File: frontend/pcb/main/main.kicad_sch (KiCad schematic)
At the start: 33 parts, among them J1 Ext, J2 Conn_01x02, J3 Conn_01x09, J4 Debug, J5 RS485, J6 Conn_01x04, J7 Conn_01x02, Q1 MMBT3904, Q2 MMBT3904, U1 ESP32-WROOM-32, U2 AP1117-33, U3 MAX485E

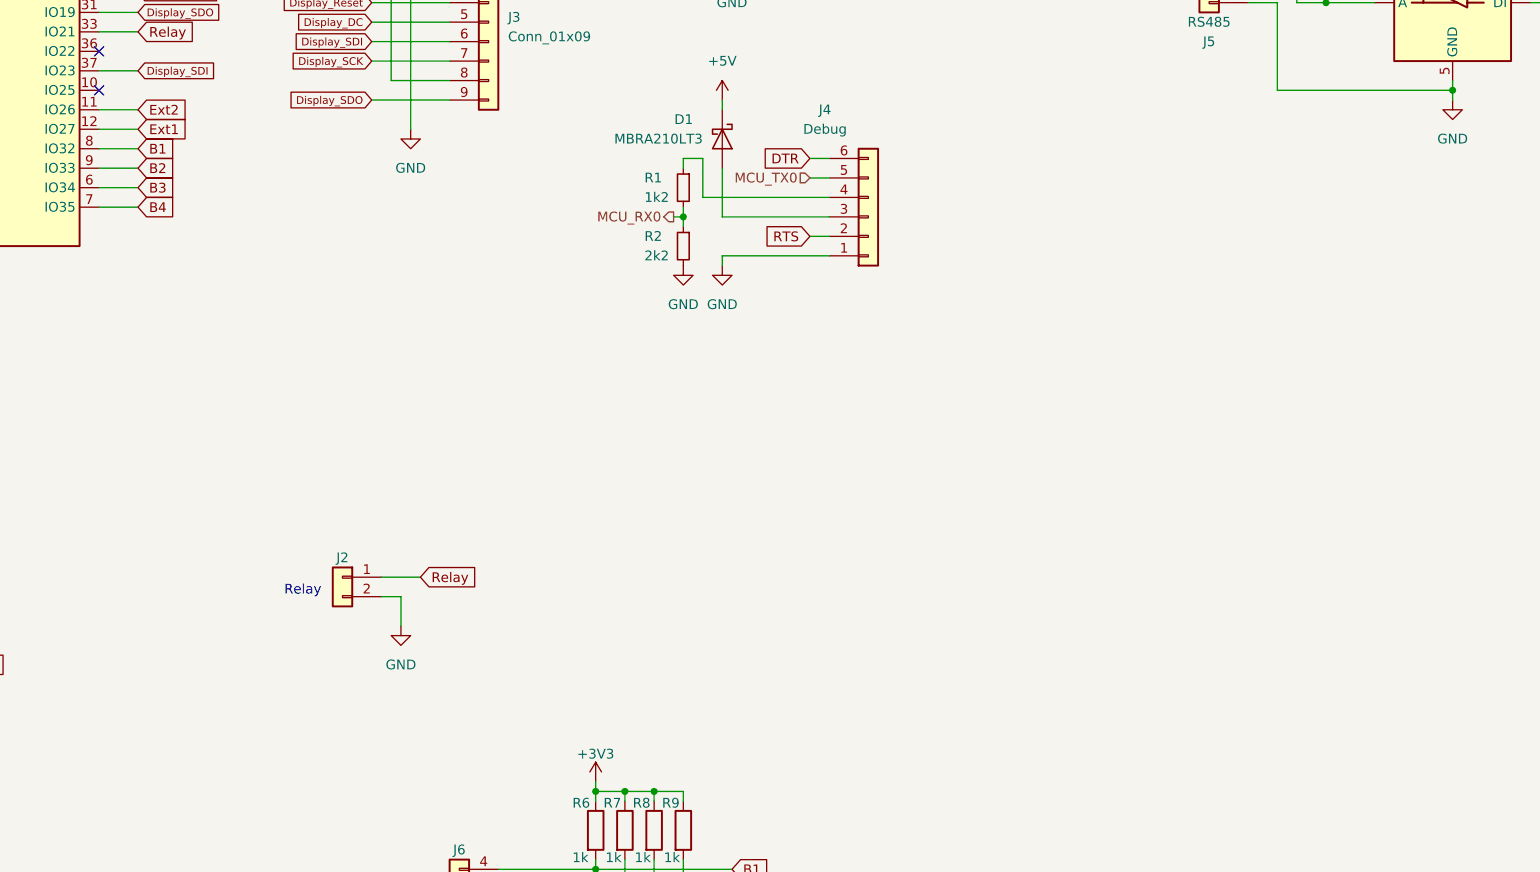
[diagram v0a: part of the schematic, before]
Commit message: Finish relay board.
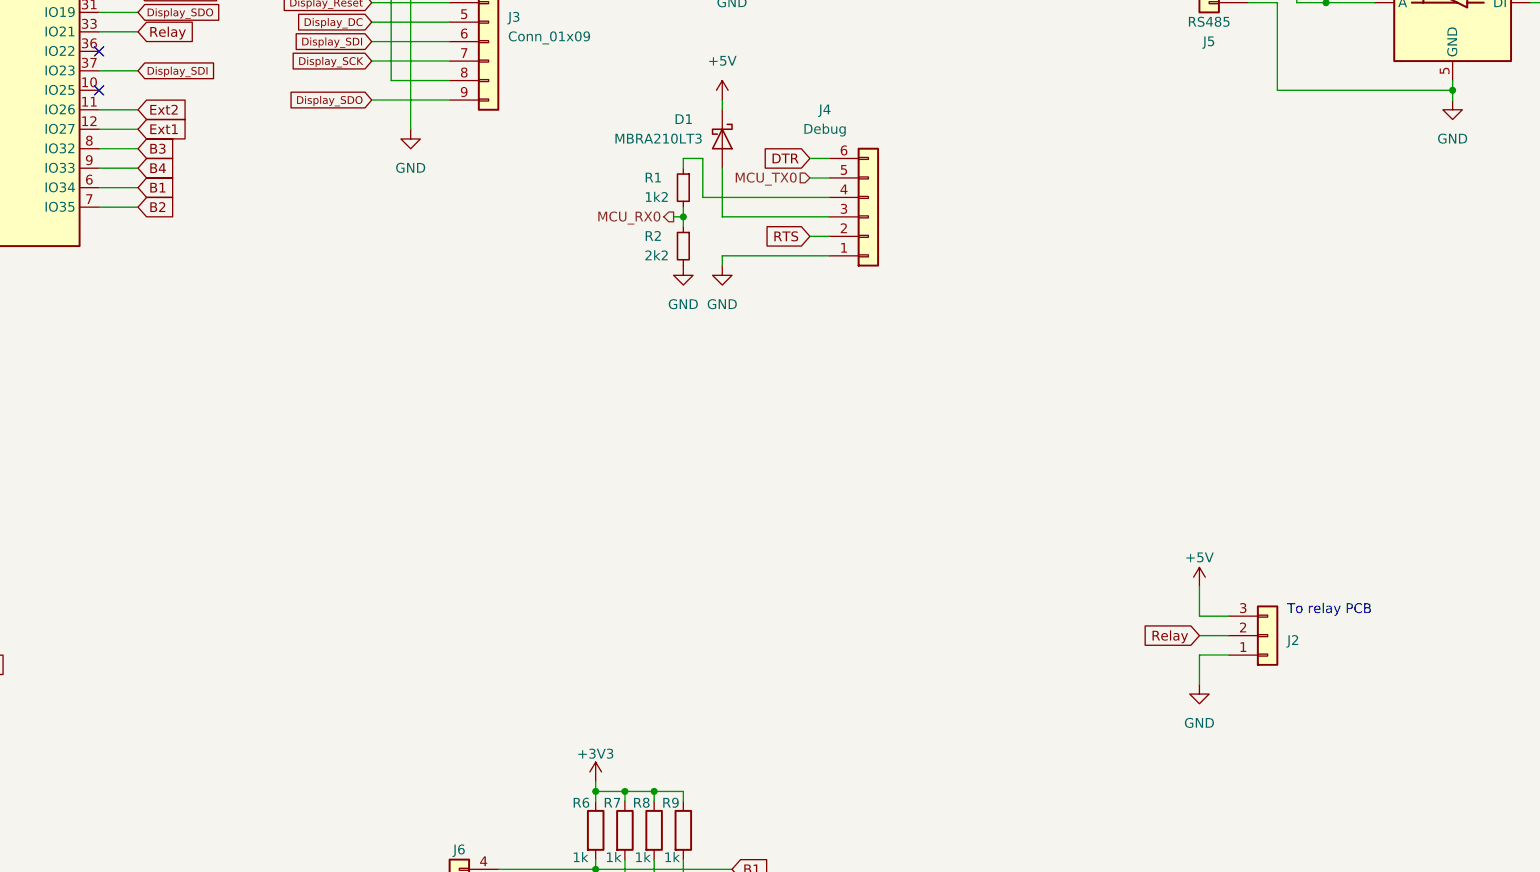
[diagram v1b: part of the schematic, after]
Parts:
- removed J2: Conn_01x02, Connector_JST:JST_XH_B2B-XH-A_1x02_P2.50mm_Vertical, symbol Connector_Generic:Conn_01x02
- added J2: Conn_01x03, Connector_PinHeader_2.54mm:PinHeader_1x03_P2.54mm_Vertical, symbol Connector_Generic:Conn_01x03
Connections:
- net +5V: now also J2.3 (Pin_3)
- net B1: now also U1.6 (IO34); no longer U1.8 (IO32)
- net B2: now also U1.7 (IO35); no longer U1.9 (IO33)
- net B3: now also U1.8 (IO32); no longer U1.6 (IO34)
- net B4: now also U1.9 (IO33); no longer U1.7 (IO35)
- net GND: now also J2.1 (Pin_1)
- net Relay: now also J2.2 (Pin_2)
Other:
- note added: "To relay PCB"
- note removed: "Relay"
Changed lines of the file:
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@@
+    (stroke (width 0) (type default))
+  )
+  (wire (pts (xy 232.41 146.05) (xy 232.41 149.86))
     (stroke (width 0) (type default))
   )
@@
     (stroke (width 0) (type default))
   )
+  (wire (pts (xy 232.41 137.16) (xy 232.41 140.97))
+    (stroke (width 0) (type default))
+  )
   (wire (pts (xy 153.67 173.99) (xy 171.45 173.99))
     (stroke (width 0) (type default))
@@
     (stroke (width 0) (type default))
   )
-  (wire (pts (xy 125.73 138.43) (xy 128.27 138.43))
-    (stroke (width 0) (type default))
-  )
   (wire (pts (xy 25.4 173.99) (xy 25.4 177.8))
     (stroke (width 0) (type default))
@@
     (stroke (width 0) (type default))
   )
-  (wire (pts (xy 128.27 138.43) (xy 128.27 142.24))
-    (stroke (width 0) (type default))
-  )
   (wire (pts (xy 88.9 46.99) (xy 93.98 46.99))
     (stroke (width 0) (type default))
   )
-  (wire (pts (xy 125.73 135.89) (xy 130.81 135.89))
-    (stroke (width 0) (type default))
-  )
   (wire (pts (xy 181.61 44.45) (xy 181.61 45.72))
     (stroke (width 0) (type default))
@@
     (stroke (width 0) (type default))
   )
+  (wire (pts (xy 232.41 143.51) (xy 236.22 143.51))
+    (stroke (width 0) (type default))
+  )
   (wire (pts (xy 58.42 147.32) (xy 68.58 147.32))
     (stroke (width 0) (type default))
@@
     (stroke (width 0) (type default))
   )
+  (wire (pts (xy 232.41 140.97) (xy 236.22 140.97))
+    (stroke (width 0) (type default))
+  )
   (wire (pts (xy 171.45 181.61) (xy 165.1 181.61))
     (stroke (width 0) (type default))
@@
     (stroke (width 0) (type default))
   )
+  (wire (pts (xy 236.22 146.05) (xy 232.41 146.05))
+    (stroke (width 0) (type default))
+  )
   (wire (pts (xy 281.94 69.85) (xy 281.94 71.12))
     (stroke (width 0) (type default))
@@
   (wire (pts (xy 88.9 31.75) (xy 91.44 31.75))
     (stroke (width 0) (type default))
-  )
-  (text "Relay" (exclude_from_sim no)
- (at 113.03 138.43 0)
-    (effects (font (size 1.27 1.27)) (justify left bottom))
   )
   (text "MSP4020" (exclude_from_sim no)
@@
     (effects (font (size 1.27 1.27)) (justify left bottom))
   )
-  (global_label "B2" (shape input) (at 93.98 82.55 0) (fields_autoplaced)
-    (effects (font (size 1.27 1.27)) (justify left))
-    (property "Intersheetrefs" "${INTERSHEET_REFS}" (at 99.3653 82.55 0)
+  (text "To relay PCB" (exclude_from_sim no)
+ (at 243.84 140.97 0)
+    (effects (font (size 1.27 1.27)) (justify left bottom))
+  )
+  (global_label "B2" (shape input) (at 93.98 87.63 0) (fields_autoplaced)
+    (effects (font (size 1.27 1.27)) (justify left))
+    (property "Intersheetrefs" "${INTERSHEET_REFS}" (at 99.3653 87.63 0)
       (effects (font (size 1.27 1.27)) (justify left) hide)
     )
@@
     )
   )
-  (global_label "B4" (shape input) (at 93.98 87.63 0) (fields_autoplaced)
-    (effects (font (size 1.27 1.27)) (justify left))
-    (property "Intersheetrefs" "${INTERSHEET_REFS}" (at 99.3653 87.63 0)
+  (global_label "B4" (shape input) (at 93.98 82.55 0) (fields_autoplaced)
+    (effects (font (size 1.27 1.27)) (justify left))
+    (property "Intersheetrefs" "${INTERSHEET_REFS}" (at 99.3653 82.55 0)
       (effects (font (size 1.27 1.27)) (justify left) hide)
     )
@@
     )
   )
-  (global_label "B3" (shape input) (at 93.98 85.09 0) (fields_autoplaced)
+  (global_label "B3" (shape input) (at 93.98 80.01 0) (fields_autoplaced)
+    (effects (font (size 1.27 1.27)) (justify left))
+    (property "Intersheetrefs" "${INTERSHEET_REFS}" (at 99.3653 80.01 0)
+      (effects (font (size 1.27 1.27)) (justify left) hide)
+    )
+  )
+  (global_label "B1" (shape input) (at 93.98 85.09 0) (fields_autoplaced)
     (effects (font (size 1.27 1.27)) (justify left))
     (property "Intersheetrefs" "${INTERSHEET_REFS}" (at 99.3653 85.09 0)
-      (effects (font (size 1.27 1.27)) (justify left) hide)
-    )
-  )
-  (global_label "B1" (shape input) (at 93.98 80.01 0) (fields_autoplaced)
-    (effects (font (size 1.27 1.27)) (justify left))
-    (property "Intersheetrefs" "${INTERSHEET_REFS}" (at 99.3653 80.01 0)
       (effects (font (size 1.27 1.27)) (justify left) hide)
     )
@@
     )
   )
-  (global_label "Relay" (shape input) (at 130.81 135.89 0) (fields_autoplaced)
-    (effects (font (size 1.27 1.27)) (justify left))
-    (property "Intersheetrefs" "${INTERSHEET_REFS}" (at 138.8562 135.89 0)
-      (effects (font (size 1.27 1.27)) (justify left) hide)
-    )
-  )
   (global_label "BOOT" (shape input) (at 91.44 29.21 0) (fields_autoplaced)
     (effects (font (size 1.27 1.27)) (justify left))
@@
     (property "Intersheetrefs" "${INTERSHEET_REFS}" (at 176.5331 178.9906 0)
       (effects (font (size 1.27 1.27)) (justify left) hide)
+    )
+  )
+  (global_label "Relay" (shape input) (at 232.41 143.51 180) (fields_autoplaced)
+    (effects (font (size 1.27 1.27)) (justify right))
+    (property "Intersheetrefs" "${INTERSHEET_REFS}" (at 224.3638 143.51 0)
+      (effects (font (size 1.27 1.27)) (justify right) hide)
     )
   )
@@
     )
   )
-  (symbol (lib_id "Connector_Generic:Conn_01x02") (at 120.65 135.89 0) (mirror y) (unit 1)
-    (in_bom yes) (on_board yes) (dnp no) (fields_autoplaced)
-    (property "Reference" "J2" (at 120.65 133.35 0)
-      (effects (font (size 1.27 1.27)))
-    )
-    (property "Value" "Conn_01x02" (at 120.65 133.35 0)
-      (effects (font (size 1.27 1.27)) hide)
-    )
-    (property "Footprint" "Connector_JST:JST_XH_B2B-XH-A_1x02_P2.50mm_Vertical" (at 120.65 135.89 0)
-      (effects (font (size 1.27 1.27)) hide)
-    )
-    (property "Datasheet" "~" (at 120.65 135.89 0)
-      (effects (font (size 1.27 1.27)) hide)
-    )
-    (pin "1")
-    (pin "2")
+  (symbol (lib_id "Connector_Generic:Conn_01x03") (at 241.3 143.51 0) (mirror x) (unit 1)
+    (in_bom yes) (on_board yes) (dnp no)
+    (property "Reference" "J2" (at 243.84 144.145 0)
+      (effects (font (size 1.27 1.27)) (justify left))
+    )
+    (property "Value" "Conn_01x03" (at 243.84 141.605 0)
+      (effects (font (size 1.27 1.27)) (justify left) hide)
+    )
+    (property "Footprint" "Connector_PinHeader_2.54mm:PinHeader_1x03_P2.54mm_Vertical" (at 241.3 143.51 0)
+      (effects (font (size 1.27 1.27)) hide)
+    )
+    (property "Datasheet" "~" (at 241.3 143.51 0)
+      (effects (font (size 1.27 1.27)) hide)
+    )
+    (pin "1")
+    (pin "2")
+    (pin "3")
     (instances
       (project "main"
@@
     )
   )
-  (symbol (lib_id "power:GND") (at 128.27 142.24 0) (unit 1)
-    (in_bom yes) (on_board yes) (dnp no) (fields_autoplaced)
-    (property "Reference" "#PWR010" (at 128.27 148.59 0)
-      (effects (font (size 1.27 1.27)) hide)
-    )
-    (property "Value" "GND" (at 128.27 147.32 0)
-      (effects (font (size 1.27 1.27)))
-    )
-    (property "Footprint" "" (at 128.27 142.24 0)
-      (effects (font (size 1.27 1.27)) hide)
-    )
-    (property "Datasheet" "" (at 128.27 142.24 0)
-      (effects (font (size 1.27 1.27)) hide)
-    )
-    (pin "1")
-    (instances
-      (project "main"
-        (path "/212a0d71-cc7b-49f8-b4ca-a935e5355dca"
-          (reference "#PWR010") (unit 1)
-        )
-      )
-    )
-  )
   (symbol (lib_id "power:+3V3") (at 33.02 33.02 0) (unit 1)
     (in_bom yes) (on_board yes) (dnp no) (fields_autoplaced)
@@
         (path "/218f1b12-ca06-4253-bcd5-950f07f2eb16"
           (reference "R9") (unit 1)
+        )
+      )
+    )
+  )
+  (symbol (lib_id "power:GND") (at 232.41 149.86 0) (unit 1)
+    (in_bom yes) (on_board yes) (dnp no) (fields_autoplaced)
+    (property "Reference" "#PWR025" (at 232.41 156.21 0)
+      (effects (font (size 1.27 1.27)) hide)
+    )
+    (property "Value" "GND" (at 232.41 154.94 0)
+      (effects (font (size 1.27 1.27)))
+    )
+    (property "Footprint" "" (at 232.41 149.86 0)
+      (effects (font (size 1.27 1.27)) hide)
+    )
+    (property "Datasheet" "" (at 232.41 149.86 0)
+      (effects (font (size 1.27 1.27)) hide)
+    )
+    (pin "1")
+    (instances
+      (project "main"
+        (path "/212a0d71-cc7b-49f8-b4ca-a935e5355dca"
+          (reference "#PWR025") (unit 1)
         )
       )
@@
         )
       )
+    )
+  )
+  (symbol (lib_id "power:+5V") (at 232.41 137.16 0) (unit 1)
+    (in_bom yes) (on_board yes) (dnp no) (fields_autoplaced)
+    (property "Reference" "#PWR024" (at 232.41 140.97 0)
+      (effects (font (size 1.27 1.27)) hide)
+    )
+    (property "Value" "+5V" (at 232.41 133.35 0)
+      (effects (font (size 1.27 1.27)))
+    )
+    (property "Footprint" "" (at 232.41 137.16 0)
+      (effects (font (size 1.27 1.27)) hide)
+    )
+    (property "Datasheet" "" (at 232.41 137.16 0)
+      (effects (font (size 1.27 1.27)) hide)
+    )
+    (pin "1")
+    (instances
+      (project "main"
+        (path "/212a0d71-cc7b-49f8-b4ca-a935e5355dca"
+          (reference "#PWR024") (unit 1)
+        )
+      )
